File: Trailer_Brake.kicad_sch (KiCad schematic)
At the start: 0 parts

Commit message: Add files via upload
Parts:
- added D146: SMBJ33A, PCM_Diode_SMD_AKL:D_SMB, symbol PCM_Diode_TVS_AKL:SMBJ33A
- added F7: Polyfuse, symbol Device:Polyfuse
- added Q52: IRLZ44N, PCM_Package_TO_SOT_THT_AKL:TO-220-3_Vertical_GDS, symbol PCM_Transistor_MOSFET_AKL:IRLZ44N
- added R200: 10k, Resistor_THT:R_Axial_DIN0207_L6.3mm_D2.5mm_P10.16mm_Horizontal, symbol PCM_SL_Resistors:10k
- added R201: .1 ohm, Resistor_THT:R_Axial_DIN0207_L6.3mm_D2.5mm_P10.16mm_Horizontal, symbol PCM_SL_Resistors:4.7k
- added R202, R203: Potentiometer, symbol Simulation_SPICE:Potentiometer
- added R204, R205: 4.7k, Resistor_THT:R_Axial_DIN0207_L6.3mm_D2.5mm_P10.16mm_Horizontal, symbol PCM_SL_Resistors:4.7k
- added SW8: SW_SPST, symbol Switch:SW_SPST
- added U14: LM339, symbol Comparator:LM339
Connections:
- new net: R202.2, U14.7 (+)
- new net: R203.2, U14.11 (+)
- new net Brake_Trailer_Shunt_Haut: Q52.3 (S), R201.2, U14.10 (-), U14.6 (-)
- new net Btn_Brake_Etat: Q52.1 (G), R200.1, SW8.2 (B)
- new net Court_Brake_Trailer: R205.1, U14.13
- new net GND: D146.2 (A), R200.2, R202.3, R203.3, U14.12 (V-), U14.5 (+), U14.9 (+)
- new net Ouvert_Brake_Trailer: R204.1, U14.1
- new net Q52.2_Drain: F7.2, Q52.2 (D)
- new net Trail_Brake: D146.1 (K), R201.1
- new net V_Arm_Trailer: F7.1
- new net V_Ref: R202.1, R203.1, R204.2, R205.2, SW8.1 (A), U14.3 (V+), U14.4 (-), U14.8 (-)
- no-connect marks 0 -> 2

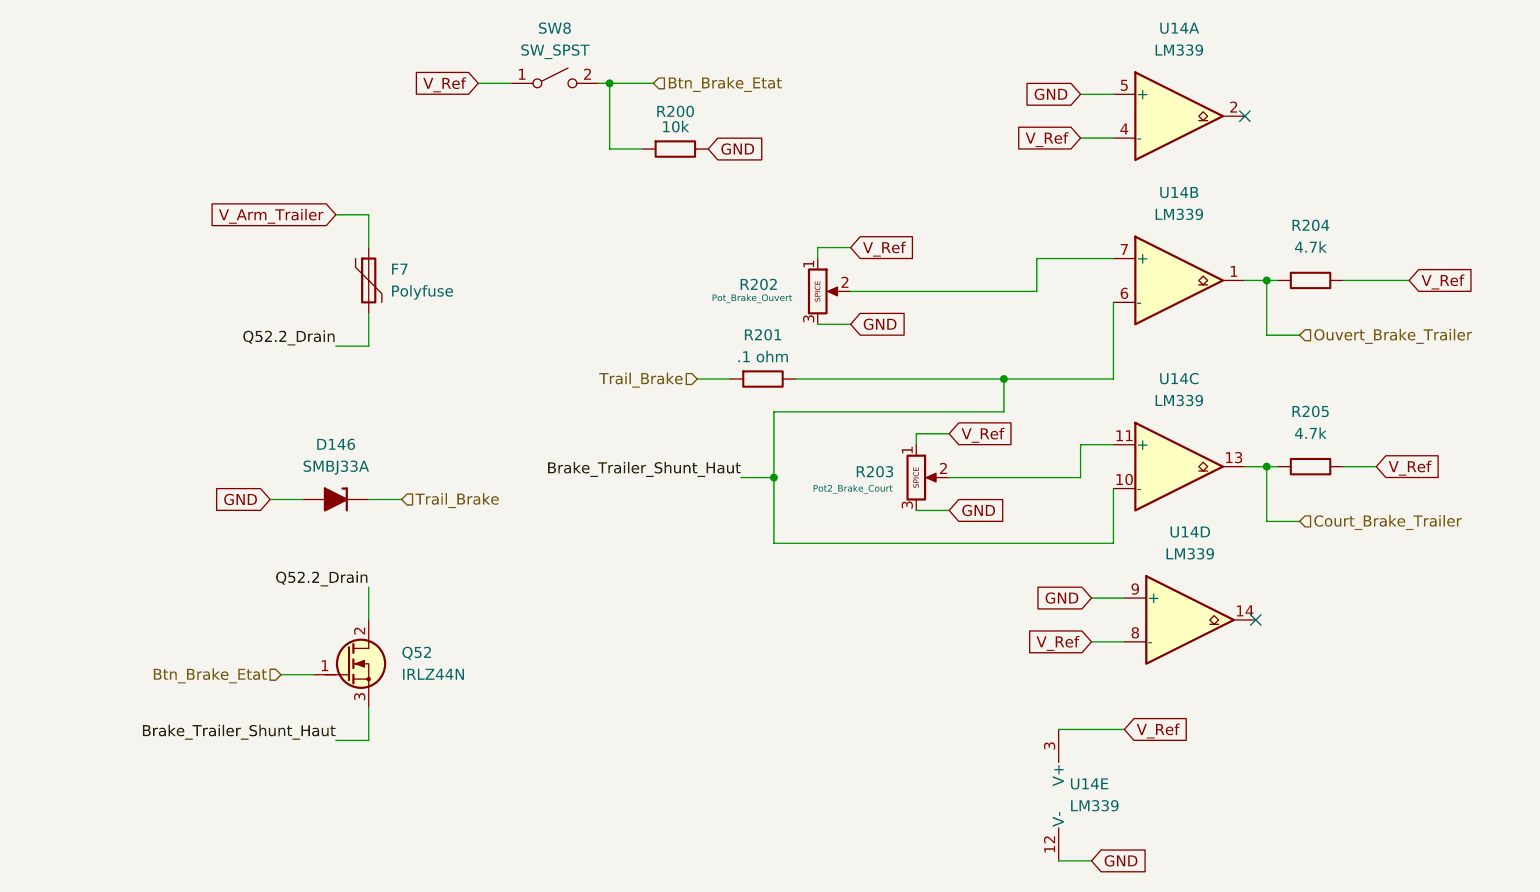
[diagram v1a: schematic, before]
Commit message: Add files via upload
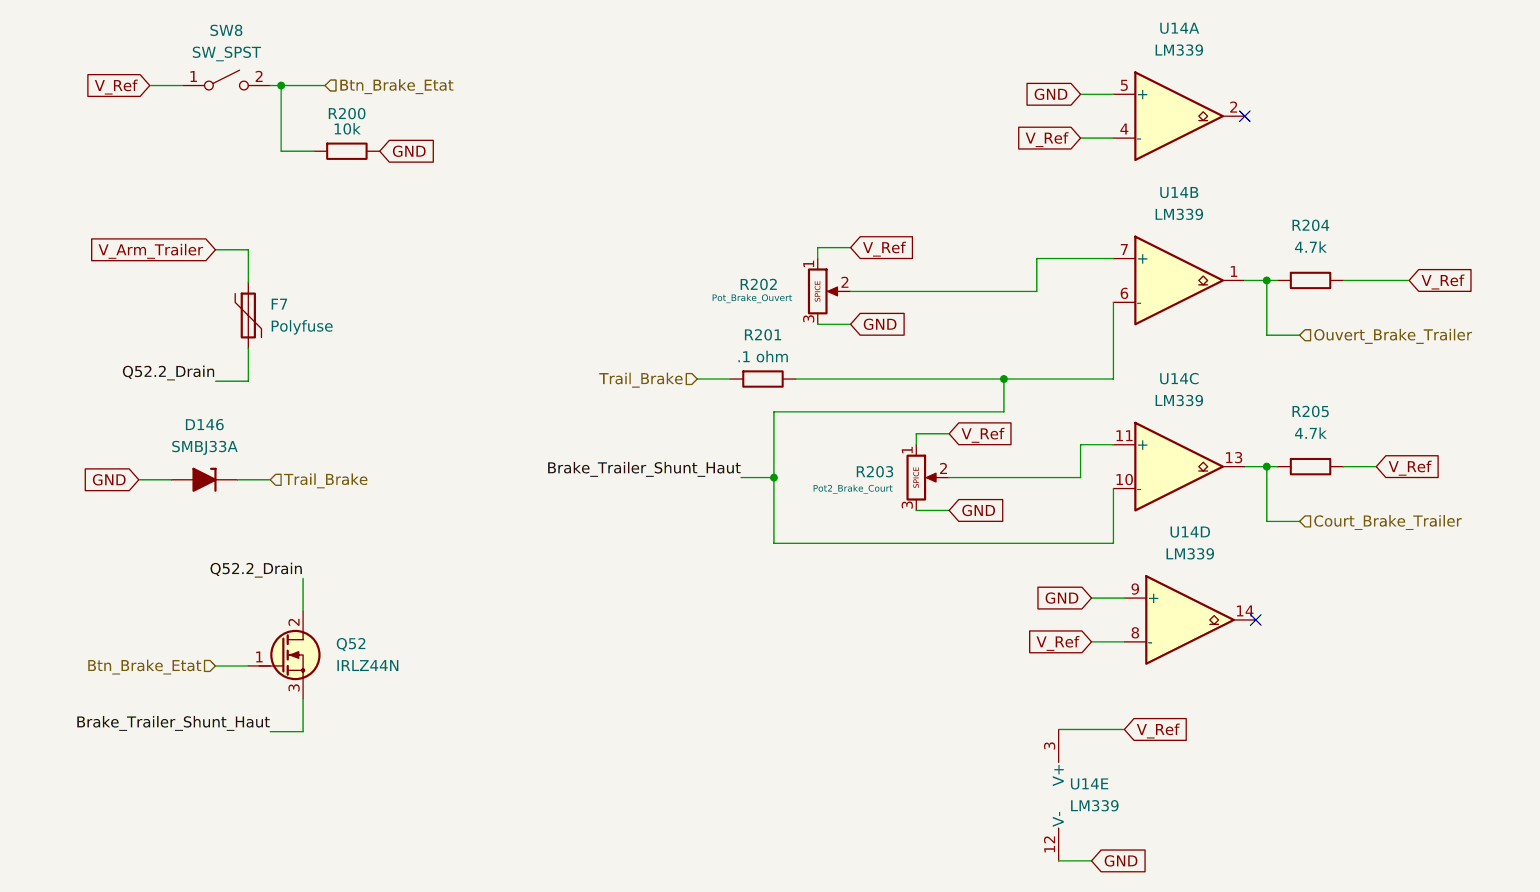
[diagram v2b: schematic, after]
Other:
- moved on the sheet: D146, F7, Q52, R200, SW8
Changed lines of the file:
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@@
 	)
 	(junction
-		(at 87.6223 27.686)
+		(at 49.53 27.94)
 		(diameter 0)
 		(color 0 0 0 0)
@@
 	(wire
 		(pts
-			(xy 49.5223 96.266) (xy 53.3323 96.266)
+			(xy 41.91 95.25) (xy 45.72 95.25)
 		)
 		(stroke
@@
 	(wire
 		(pts
-			(xy 87.6223 27.686) (xy 87.6223 35.306)
-		)
-		(stroke
-			(width 0)
-			(type default)
-		)
-	)
-	(wire
-		(pts
-			(xy 48.2523 75.946) (xy 52.0623 75.946)
+			(xy 49.53 27.94) (xy 49.53 35.56)
+		)
+		(stroke
+			(width 0)
+			(type default)
+		)
+	)
+	(wire
+		(pts
+			(xy 33.02 73.66) (xy 36.83 73.66)
 		)
 		(stroke
@@
 	(wire
 		(pts
-			(xy 59.6823 86.106) (xy 59.6823 89.916)
+			(xy 52.07 85.09) (xy 52.07 88.9)
 		)
 		(stroke
@@
 	(wire
 		(pts
-			(xy 55.8723 58.166) (xy 59.6823 58.166)
+			(xy 41.91 62.23) (xy 45.72 62.23)
 		)
 		(stroke
@@
 	(wire
 		(pts
-			(xy 55.8723 42.926) (xy 59.6823 42.926)
+			(xy 41.91 46.99) (xy 45.72 46.99)
 		)
 		(stroke
@@
 	(wire
 		(pts
-			(xy 92.7023 27.686) (xy 87.6223 27.686)
-		)
-		(stroke
-			(width 0)
-			(type default)
-		)
-	)
-	(wire
-		(pts
-			(xy 86.3523 27.686) (xy 87.6223 27.686)
+			(xy 54.61 27.94) (xy 49.53 27.94)
+		)
+		(stroke
+			(width 0)
+			(type default)
+		)
+	)
+	(wire
+		(pts
+			(xy 48.26 27.94) (xy 49.53 27.94)
 		)
 		(stroke
@@
 	(wire
 		(pts
-			(xy 87.6223 35.306) (xy 91.4323 35.306)
+			(xy 49.53 35.56) (xy 53.34 35.56)
 		)
 		(stroke
@@
 	(wire
 		(pts
-			(xy 59.6823 54.356) (xy 59.6823 58.166)
-		)
-		(stroke
-			(width 0)
-			(type default)
-		)
-	)
-	(wire
-		(pts
-			(xy 72.3823 27.686) (xy 76.1923 27.686)
+			(xy 45.72 58.42) (xy 45.72 62.23)
+		)
+		(stroke
+			(width 0)
+			(type default)
+		)
+	)
+	(wire
+		(pts
+			(xy 34.29 27.94) (xy 38.1 27.94)
 		)
 		(stroke
@@
 	(wire
 		(pts
-			(xy 59.6823 42.926) (xy 59.6823 46.736)
+			(xy 45.72 46.99) (xy 45.72 50.8)
 		)
 		(stroke
@@
 	(wire
 		(pts
-			(xy 59.6823 75.946) (xy 63.4923 75.946)
+			(xy 44.45 73.66) (xy 48.26 73.66)
 		)
 		(stroke
@@
 	(wire
 		(pts
-			(xy 59.6823 100.076) (xy 59.6823 103.886)
+			(xy 52.07 99.06) (xy 52.07 102.87)
 		)
 		(stroke
@@
 	(wire
 		(pts
-			(xy 55.8723 103.886) (xy 59.6823 103.886)
+			(xy 48.26 102.87) (xy 52.07 102.87)
 		)
 		(stroke
@@
 	)
 	(label "Q52.2_Drain"
-		(at 59.6823 86.106 180)
+		(at 52.07 85.09 180)
 		(effects
 			(font
@@
 	)
 	(label "Q52.2_Drain"
-		(at 55.8723 58.166 180)
+		(at 41.91 62.23 180)
 		(effects
 			(font
@@
 	)
 	(label "Brake_Trailer_Shunt_Haut"
-		(at 55.8723 103.886 180)
+		(at 48.26 102.87 180)
 		(effects
 			(font
@@
 	(global_label "GND"
 		(shape input)
-		(at 99.0523 35.306 0)
+		(at 60.96 35.56 0)
 		(fields_autoplaced yes)
 		(effects
@@
 		)
 		(property "Intersheetrefs" "${INTERSHEET_REFS}"
-			(at 105.908 35.306 0)
+			(at 67.8157 35.56 0)
 			(hide yes)
 			(show_name no)
@@
 	(global_label "GND"
 		(shape input)
-		(at 48.2523 75.946 180)
+		(at 33.02 73.66 180)
 		(fields_autoplaced yes)
 		(effects
@@
 		)
 		(property "Intersheetrefs" "${INTERSHEET_REFS}"
-			(at 41.3966 75.946 0)
+			(at 26.1643 73.66 0)
 			(hide yes)
 			(show_name no)
@@
 	(global_label "V_Ref"
 		(shape input)
-		(at 72.3823 27.686 180)
+		(at 34.29 27.94 180)
 		(fields_autoplaced yes)
 		(effects
@@
 		)
 		(property "Intersheetrefs" "${INTERSHEET_REFS}"
-			(at 64.2566 27.686 0)
+			(at 26.1643 27.94 0)
 			(hide yes)
 			(show_name no)
@@
 	(global_label "V_Arm_Trailer"
 		(shape input)
-		(at 55.8723 42.926 180)
+		(at 41.91 46.99 180)
 		(fields_autoplaced yes)
 		(effects
@@
 		)
 		(property "Intersheetrefs" "${INTERSHEET_REFS}"
-			(at 40.2476 42.926 0)
+			(at 26.2853 46.99 0)
 			(hide yes)
 			(show_name no)
@@
 	(hierarchical_label "Btn_Brake_Etat"
 		(shape input)
-		(at 49.5223 96.266 180)
+		(at 41.91 95.25 180)
 		(effects
 			(font
@@
 	(hierarchical_label "Btn_Brake_Etat"
 		(shape input)
-		(at 92.7023 27.686 0)
+		(at 54.61 27.94 0)
 		(effects
 			(font
@@
 	(hierarchical_label "Trail_Brake"
 		(shape input)
-		(at 63.4923 75.946 0)
+		(at 48.26 73.66 0)
 		(effects
 			(font
@@
 	(symbol
 		(lib_id "PCM_SL_Resistors:10k")
-		(at 95.2423 35.306 0)
+		(at 57.15 35.56 0)
 		(unit 1)
 		(body_style 1)
@@
 		(dnp no)
 		(property "Reference" "R200"
-			(at 95.2423 30.988 0)
+			(at 57.15 31.242 0)
 			(show_name no)
 			(do_not_autoplace no)
@@
 		)
 		(property "Value" "10k"
-			(at 95.2423 32.766 0)
+			(at 57.15 33.02 0)
 			(show_name no)
 			(do_not_autoplace no)
@@
 		)
 		(property "Footprint" "Resistor_THT:R_Axial_DIN0207_L6.3mm_D2.5mm_P10.16mm_Horizontal"
-			(at 96.1313 39.624 0)
+			(at 58.039 39.878 0)
 			(hide yes)
 			(show_name no)
@@
 		)
 		(property "Datasheet" ""
-			(at 95.7503 35.306 0)
+			(at 57.658 35.56 0)
 			(hide yes)
 			(show_name no)
@@
 		)
 		(property "Description" "10kΩ, 1/4W Resistor"
-			(at 95.2423 35.306 0)
+			(at 57.15 35.56 0)
 			(hide yes)
 			(show_name no)
@@
 	(symbol
 		(lib_id "PCM_Diode_TVS_AKL:SMBJ33A")
-		(at 55.8723 75.946 0)
+		(at 40.64 73.66 0)
 		(unit 1)
 		(body_style 1)
@@
 		(fields_autoplaced yes)
 		(property "Reference" "D146"
-			(at 55.8723 69.596 0)
+			(at 40.64 67.31 0)
 			(show_name no)
 			(do_not_autoplace no)
@@
 		)
 		(property "Value" "SMBJ33A"
-			(at 55.8723 72.136 0)
+			(at 40.64 69.85 0)
 			(show_name no)
 			(do_not_autoplace no)
@@
 		)
 		(property "Footprint" "PCM_Diode_SMD_AKL:D_SMB"
-			(at 55.8723 75.946 0)
+			(at 40.64 73.66 0)
 			(hide yes)
 			(show_name no)
@@
 		)
 		(property "Datasheet" "https://www.tme.eu/Document/0b6222bec7e12d83185b51d73cb6a54d/SMBJ_ser.pdf"
-			(at 55.8723 75.946 0)
+			(at 40.64 73.66 0)
 			(hide yes)
 			(show_name no)
@@
 		)
 		(property "Description" "SMB Unidirectional TVS diode, 33V, 600W, Alternate KiCAD Library"
-			(at 55.8723 75.946 0)
+			(at 40.64 73.66 0)
 			(hide yes)
 			(show_name no)
@@
 	(symbol
 		(lib_id "PCM_Transistor_MOSFET_AKL:IRLZ44N")
-		(at 57.1423 94.996 0)
+		(at 49.53 93.98 0)
 		(unit 1)
 		(body_style 1)
@@
 		(fields_autoplaced yes)
 		(property "Reference" "Q52"
-			(at 63.4923 93.7259 0)
+			(at 55.88 92.7099 0)
 			(show_name no)
 			(do_not_autoplace no)
@@
 		)
 		(property "Value" "IRLZ44N"
-			(at 63.4923 96.2659 0)
+			(at 55.88 95.2499 0)
 			(show_name no)
 			(do_not_autoplace no)
@@
 		)
 		(property "Footprint" "PCM_Package_TO_SOT_THT_AKL:TO-220-3_Vertical_GDS"
-			(at 62.2223 92.456 0)
+			(at 54.61 91.44 0)
 			(hide yes)
 			(show_name no)
@@
 		)
 		(property "Datasheet" "https://www.tme.eu/Document/71cf1899624764088671ce6de5d15eb4/irlz44n.pdf"
-			(at 57.1423 94.996 0)
+			(at 49.53 93.98 0)
 			(hide yes)
 			(show_name no)
@@
 		)
 		(property "Description" "TO-220 N-MOSFET enchancement mode transistor, 55V, 47A, 110W, Alternate KiCAD Library"
-			(at 57.1423 94.996 0)
+			(at 49.53 93.98 0)
 			(hide yes)
 			(show_name no)
@@
 	(symbol
 		(lib_id "Device:Polyfuse")
-		(at 59.6823 50.546 0)
+		(at 45.72 54.61 0)
 		(unit 1)
 		(body_style 1)
@@
 		(fields_autoplaced yes)
 		(property "Reference" "F7"
-			(at 62.2223 49.2759 0)
+			(at 48.26 53.3399 0)
 			(show_name no)
 			(do_not_autoplace no)
@@
 		)
 		(property "Value" "Polyfuse"
-			(at 62.2223 51.8159 0)
+			(at 48.26 55.8799 0)
 			(show_name no)
 			(do_not_autoplace no)
@@
 		)
 		(property "Footprint" ""
-			(at 60.9523 55.626 0)
+			(at 46.99 59.69 0)
 			(hide yes)
 			(show_name no)
@@
 		)
 		(property "Datasheet" ""
-			(at 59.6823 50.546 0)
+			(at 45.72 54.61 0)
 			(hide yes)
 			(show_name no)
@@
 		)
 		(property "Description" "Resettable fuse, polymeric positive temperature coefficient"
-			(at 59.6823 50.546 0)
+			(at 45.72 54.61 0)
 			(hide yes)
 			(show_name no)
@@
 	(symbol
 		(lib_id "Switch:SW_SPST")
-		(at 81.2723 27.686 0)
+		(at 43.18 27.94 0)
 		(unit 1)
 		(body_style 1)
@@
 		(fields_autoplaced yes)
 		(property "Reference" "SW8"
-			(at 81.2723 21.336 0)
+			(at 43.18 21.59 0)
 			(show_name no)
 			(do_not_autoplace no)
@@
 		)
 		(property "Value" "SW_SPST"
-			(at 81.2723 23.876 0)
+			(at 43.18 24.13 0)
 			(show_name no)
 			(do_not_autoplace no)
@@
 		)
 		(property "Footprint" ""
-			(at 81.2723 27.686 0)
+			(at 43.18 27.94 0)
 			(hide yes)
 			(show_name no)
@@
 		)
 		(property "Datasheet" ""
-			(at 81.2723 27.686 0)
+			(at 43.18 27.94 0)
 			(hide yes)
 			(show_name no)
@@
 		)
 		(property "Description" "Single Pole Single Throw (SPST) switch"
-			(at 81.2723 27.686 0)
-			(hide yes)
-			(show_name no)
+			(at 43.18 27.94 0)
+			(hide yes)
+			(show_name no)

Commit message: Add files via upload
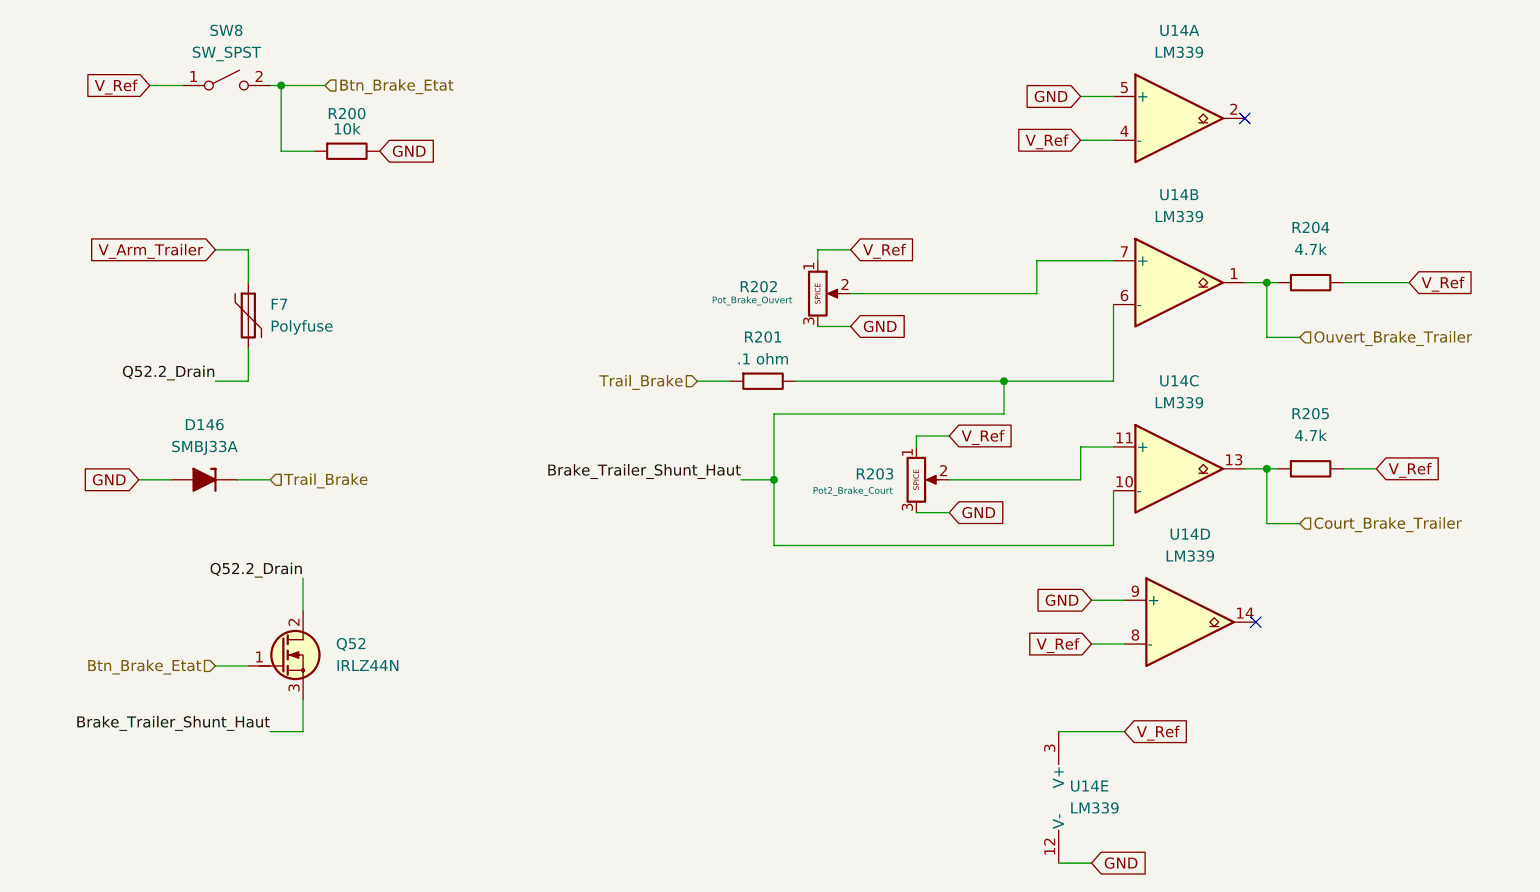
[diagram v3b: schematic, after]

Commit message: Add files via upload
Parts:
- R201: footprint Resistor_THT:R_Axial_DIN0207_L6.3mm_D2.5mm_P10.16mm_Horizontal -> Resistor_THT:R_Axial_Power_L25.0mm_W9.0mm_P27.94mm
- R202, R203: footprint (none) -> TRIM_3296W1103LF:TRIM_3296W1103LF
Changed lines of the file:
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@@
 			)
 		)
-		(property "Footprint" ""
+		(property "Footprint" "TRIM_3296W1103LF:TRIM_3296W1103LF"
 			(at 111.76 52.07 0)
 			(hide yes)
@@
 			)
 		)
-		(property "Footprint" "Resistor_THT:R_Axial_DIN0207_L6.3mm_D2.5mm_P10.16mm_Horizontal"
+		(property "Footprint" "Resistor_THT:R_Axial_Power_L25.0mm_W9.0mm_P27.94mm"
 			(at 106.299 66.548 0)
 			(hide yes)
@@
 			)
 		)
-		(property "Footprint" ""
+		(property "Footprint" "TRIM_3296W1103LF:TRIM_3296W1103LF"
 			(at 123.19 73.66 0)
 			(hide yes)

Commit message: Add files via upload
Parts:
- U14: footprint (none) -> Package_DIP:DIP-14_W7.62mm_Socket
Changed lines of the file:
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@@
 			)
 		)
-		(property "Footprint" ""
+		(property "Footprint" "Package_DIP:DIP-14_W7.62mm_Socket"
 			(at 153.67 87.63 0)
 			(hide yes)
@@
 			)
 		)
-		(property "Footprint" ""
+		(property "Footprint" "Package_DIP:DIP-14_W7.62mm_Socket"
 			(at 152.4 29.21 0)
 			(hide yes)
@@
 			)
 		)
-		(property "Footprint" ""
+		(property "Footprint" "Package_DIP:DIP-14_W7.62mm_Socket"
 			(at 140.97 107.95 0)
 			(hide yes)
@@
 			)
 		)
-		(property "Footprint" ""
+		(property "Footprint" "Package_DIP:DIP-14_W7.62mm_Socket"
 			(at 152.4 48.26 0)
 			(hide yes)
@@
 			)
 		)
-		(property "Footprint" ""
+		(property "Footprint" "Package_DIP:DIP-14_W7.62mm_Socket"
 			(at 152.4 69.85 0)
 			(hide yes)

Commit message: Add files via upload
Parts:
- U14: footprint Package_DIP:DIP-14_W7.62mm_Socket -> (none)
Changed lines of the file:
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@@
 			)
 		)
-		(property "Footprint" "Package_DIP:DIP-14_W7.62mm_Socket"
+		(property "Footprint" ""
 			(at 153.67 87.63 0)
 			(hide yes)
@@
 			)
 		)
-		(property "Footprint" "Package_DIP:DIP-14_W7.62mm_Socket"
+		(property "Footprint" ""
 			(at 152.4 29.21 0)
 			(hide yes)
@@
 			)
 		)
-		(property "Footprint" "Package_DIP:DIP-14_W7.62mm_Socket"
+		(property "Footprint" ""
 			(at 140.97 107.95 0)
 			(hide yes)
@@
 			)
 		)
-		(property "Footprint" "Package_DIP:DIP-14_W7.62mm_Socket"
+		(property "Footprint" ""
 			(at 152.4 48.26 0)
 			(hide yes)
@@
 			)
 		)
-		(property "Footprint" "Package_DIP:DIP-14_W7.62mm_Socket"
+		(property "Footprint" ""
 			(at 152.4 69.85 0)
 			(hide yes)

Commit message: Add files via upload
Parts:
- R201: footprint Resistor_THT:R_Axial_Power_L25.0mm_W9.0mm_P27.94mm -> Resistor_THT:R_Axial_DIN0207_L6.3mm_D2.5mm_P10.16mm_Horizontal
- R202, R203: footprint TRIM_3296W1103LF:TRIM_3296W1103LF -> (none)
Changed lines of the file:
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@@
 			)
 		)
-		(property "Footprint" "TRIM_3296W1103LF:TRIM_3296W1103LF"
+		(property "Footprint" ""
 			(at 111.76 52.07 0)
 			(hide yes)
@@
 			)
 		)
-		(property "Footprint" "Resistor_THT:R_Axial_Power_L25.0mm_W9.0mm_P27.94mm"
+		(property "Footprint" "Resistor_THT:R_Axial_DIN0207_L6.3mm_D2.5mm_P10.16mm_Horizontal"
 			(at 106.299 66.548 0)
 			(hide yes)
@@
 			)
 		)
-		(property "Footprint" "TRIM_3296W1103LF:TRIM_3296W1103LF"
+		(property "Footprint" ""
 			(at 123.19 73.66 0)
 			(hide yes)

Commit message: Add files via upload
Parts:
- R201: footprint Resistor_THT:R_Axial_DIN0207_L6.3mm_D2.5mm_P10.16mm_Horizontal -> PCM_SL_Devices:Resistor_5W
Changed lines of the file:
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@@
 			)
 		)
-		(property "Footprint" "Resistor_THT:R_Axial_DIN0207_L6.3mm_D2.5mm_P10.16mm_Horizontal"
+		(property "Footprint" "PCM_SL_Devices:Resistor_5W"
 			(at 106.299 66.548 0)
 			(hide yes)
